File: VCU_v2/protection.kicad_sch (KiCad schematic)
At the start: 8 parts, among them Q1 PMOS

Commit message: bspd schematic done
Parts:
- D7: LCSC P/N (none) -> C99290
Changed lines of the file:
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@@
+			)
+		)
+		(property "LCSC P/N" "C99290"
+			(at 147.32 68.58 90)
+			(effects
+				(font
+					(size 1.27 1.27)
+				)
+				(hide yes)
 			)
 		)

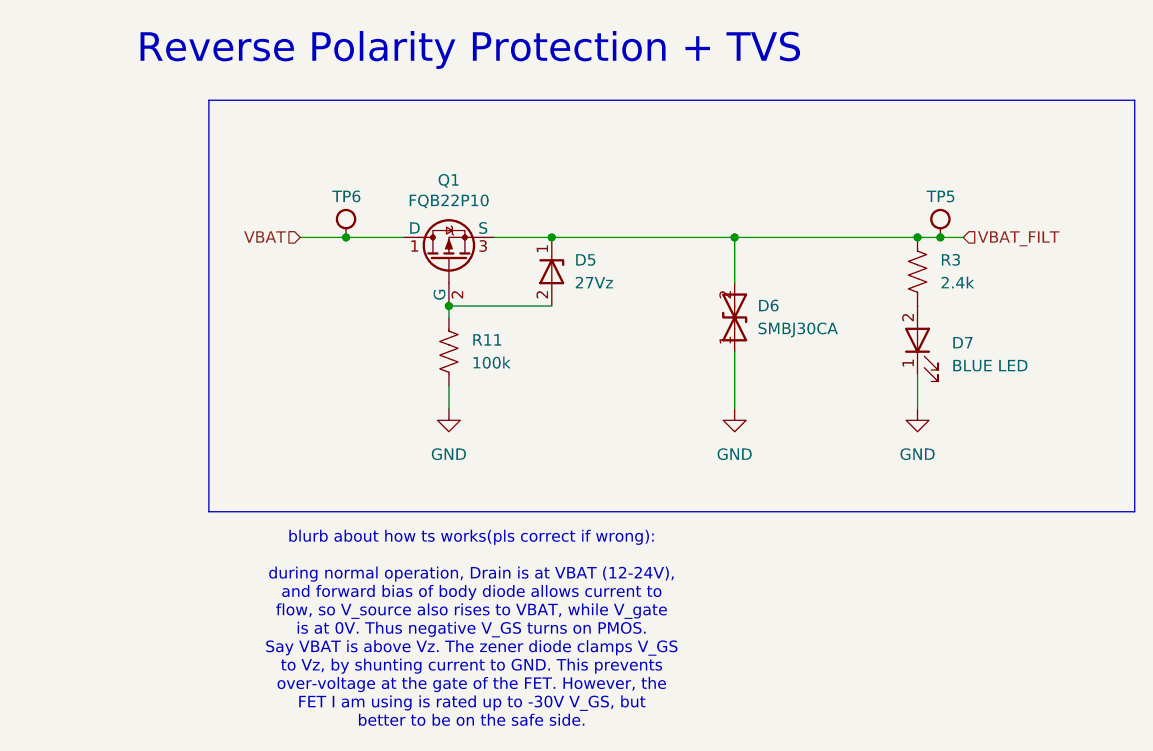
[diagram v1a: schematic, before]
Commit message: vcu v2 schematics done
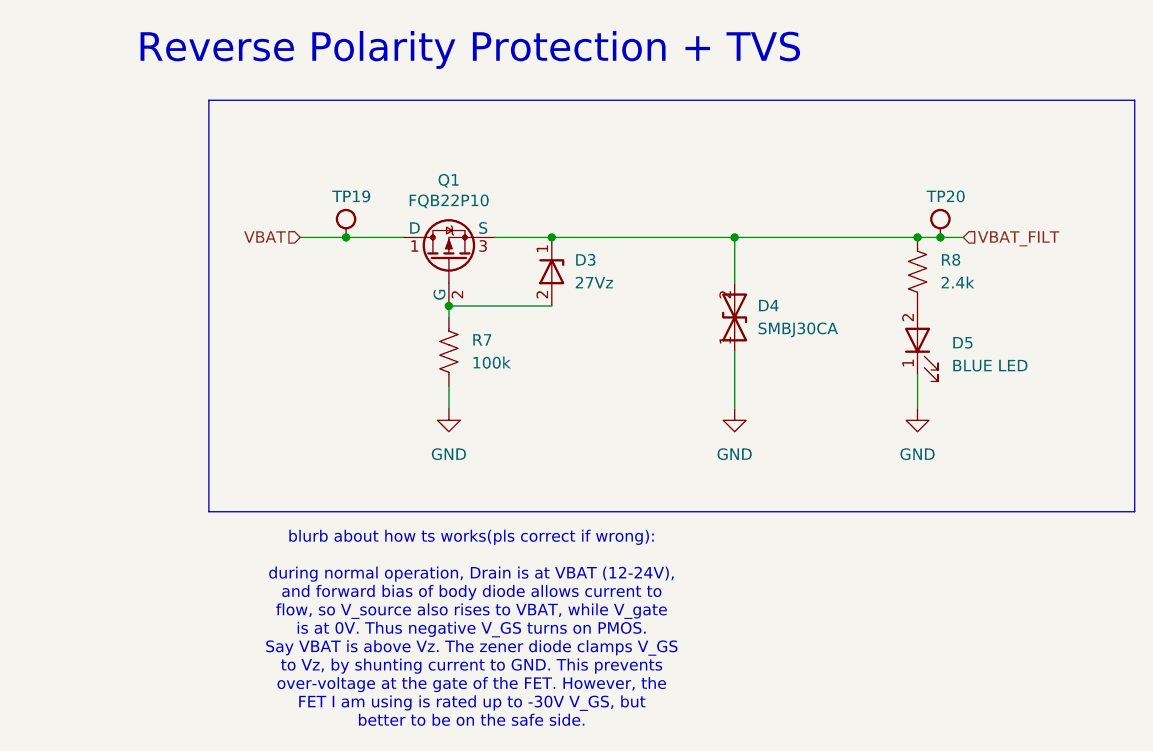
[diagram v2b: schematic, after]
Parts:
- renumbered D5 to D3, D6 to D4, D7 to D5, R11 to R7, R3 to R8, TP6 to TP19, TP5 to TP20
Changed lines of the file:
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@@
 		(dnp no)
 		(fields_autoplaced yes)
-		(property "Reference" "D5"
+		(property "Reference" "D3"
 			(at 109.22 59.6899 90)
 			(effects
@@
 			(project ""
 				(path "/4ee6c2ad-9a1b-4276-b3cf-1cc8dc52967e/9e4b5f8d-93dc-46d5-aa92-d0e0d2e07b3d/b7d8a0a7-c635-4617-919c-9464d63ae6b1"
-					(reference "D5")
+					(reference "D3")
 					(unit 1)
 				)
@@
 		(on_board yes)
 		(dnp no)
-		(property "Reference" "TP5"
+		(property "Reference" "TP20"
 			(at 148.3368 51.8937 0)
 			(effects
@@
 			(project "VCU_v1"
 				(path "/4ee6c2ad-9a1b-4276-b3cf-1cc8dc52967e/9e4b5f8d-93dc-46d5-aa92-d0e0d2e07b3d/b7d8a0a7-c635-4617-919c-9464d63ae6b1"
-					(reference "TP5")
+					(reference "TP20")
 					(unit 1)
 				)
@@
 		(on_board yes)
 		(dnp no)
-		(property "Reference" "TP6"
+		(property "Reference" "TP19"
 			(at 82.2968 51.8937 0)
 			(effects
@@
 			(project "VCU_v1"
 				(path "/4ee6c2ad-9a1b-4276-b3cf-1cc8dc52967e/9e4b5f8d-93dc-46d5-aa92-d0e0d2e07b3d/b7d8a0a7-c635-4617-919c-9464d63ae6b1"
-					(reference "TP6")
+					(reference "TP19")
 					(unit 1)
 				)
@@
 		(dnp no)
 		(fields_autoplaced yes)
-		(property "Reference" "#PWR059"
+		(property "Reference" "#PWR039"
 			(at 127 82.55 0)
 			(effects
@@
 			(project "VCU_v1"
 				(path "/4ee6c2ad-9a1b-4276-b3cf-1cc8dc52967e/9e4b5f8d-93dc-46d5-aa92-d0e0d2e07b3d/b7d8a0a7-c635-4617-919c-9464d63ae6b1"
-					(reference "#PWR059")
+					(reference "#PWR039")
 					(unit 1)
 				)
@@
 		(dnp no)
 		(fields_autoplaced yes)
-		(property "Reference" "D7"
+		(property "Reference" "D5"
 			(at 151.13 68.8974 90)
 			(effects
@@
 			(project ""
 				(path "/4ee6c2ad-9a1b-4276-b3cf-1cc8dc52967e/9e4b5f8d-93dc-46d5-aa92-d0e0d2e07b3d/b7d8a0a7-c635-4617-919c-9464d63ae6b1"
-					(reference "D7")
+					(reference "D5")
 					(unit 1)
 				)
@@
 		(dnp no)
 		(fields_autoplaced yes)
-		(property "Reference" "R11"
+		(property "Reference" "R7"
 			(at 97.79 68.5799 90)
 			(effects
@@
 			(project ""
 				(path "/4ee6c2ad-9a1b-4276-b3cf-1cc8dc52967e/9e4b5f8d-93dc-46d5-aa92-d0e0d2e07b3d/b7d8a0a7-c635-4617-919c-9464d63ae6b1"
-					(reference "R11")
+					(reference "R7")
 					(unit 1)
 				)
@@
 		(dnp no)
 		(fields_autoplaced yes)
-		(property "Reference" "D6"
+		(property "Reference" "D4"
 			(at 129.54 64.7699 90)
 			(effects
@@
 			(project ""
 				(path "/4ee6c2ad-9a1b-4276-b3cf-1cc8dc52967e/9e4b5f8d-93dc-46d5-aa92-d0e0d2e07b3d/b7d8a0a7-c635-4617-919c-9464d63ae6b1"
-					(reference "D6")
+					(reference "D4")
 					(unit 1)
 				)
@@
 		(dnp no)
 		(fields_autoplaced yes)
-		(property "Reference" "#PWR058"
+		(property "Reference" "#PWR038"
 			(at 95.25 82.55 0)
 			(effects
@@
 			(project ""
 				(path "/4ee6c2ad-9a1b-4276-b3cf-1cc8dc52967e/9e4b5f8d-93dc-46d5-aa92-d0e0d2e07b3d/b7d8a0a7-c635-4617-919c-9464d63ae6b1"
-					(reference "#PWR058")
+					(reference "#PWR038")
 					(unit 1)
 				)
@@
 		(dnp no)
 		(fields_autoplaced yes)
-		(property "Reference" "R3"
+		(property "Reference" "R8"
 			(at 149.86 59.6899 90)
 			(effects
@@
 			(project ""
 				(path "/4ee6c2ad-9a1b-4276-b3cf-1cc8dc52967e/9e4b5f8d-93dc-46d5-aa92-d0e0d2e07b3d/b7d8a0a7-c635-4617-919c-9464d63ae6b1"
-					(reference "R3")
+					(reference "R8")
 					(unit 1)
 				)
@@
 		(dnp no)
 		(fields_autoplaced yes)
-		(property "Reference" "#PWR060"
+		(property "Reference" "#PWR040"
 			(at 147.32 82.55 0)
 			(effects
@@
 			(project ""
 				(path "/4ee6c2ad-9a1b-4276-b3cf-1cc8dc52967e/9e4b5f8d-93dc-46d5-aa92-d0e0d2e07b3d/b7d8a0a7-c635-4617-919c-9464d63ae6b1"
-					(reference "#PWR060")
+					(reference "#PWR040")
 					(unit 1)
 				)

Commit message: placements friggin 80% friggin done shoutout epstein
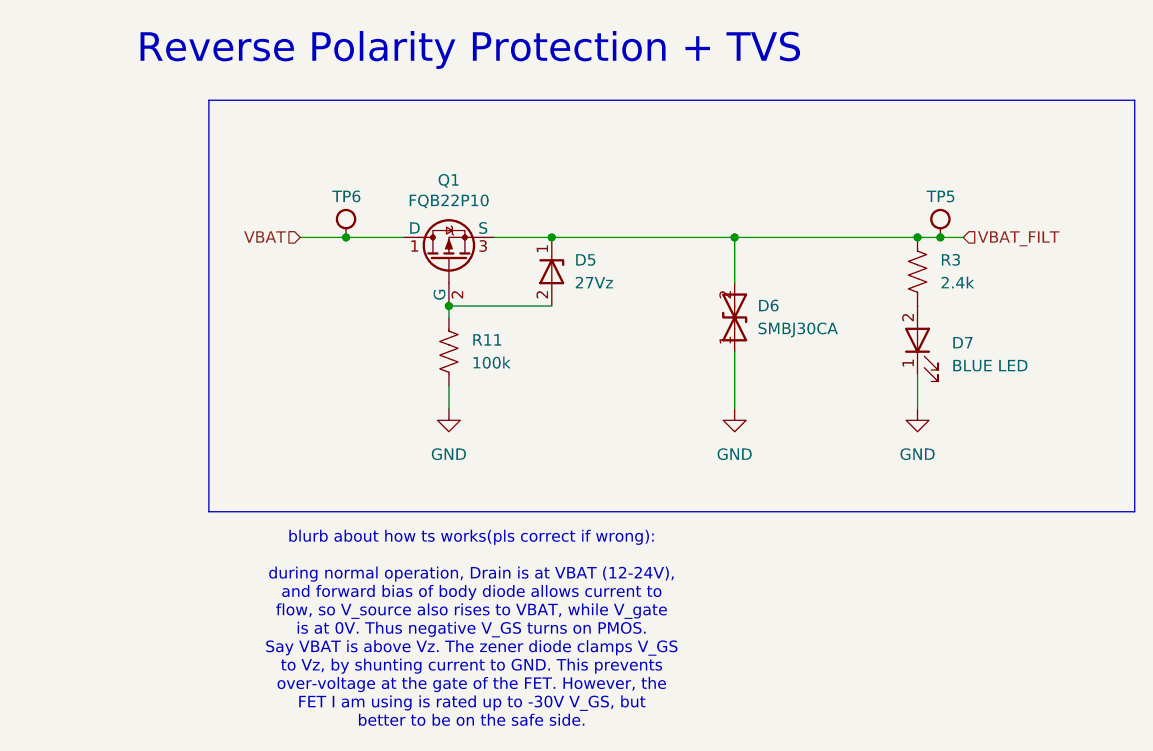
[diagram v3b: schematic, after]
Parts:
- renumbered D3 to D5, D4 to D6, D5 to D7, R7 to R11, R8 to R3, TP20 to TP5, TP19 to TP6
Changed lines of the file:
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@@
 		(dnp no)
 		(fields_autoplaced yes)
-		(property "Reference" "D3"
+		(property "Reference" "D5"
 			(at 109.22 59.6899 90)
 			(effects
@@
 			(project ""
 				(path "/4ee6c2ad-9a1b-4276-b3cf-1cc8dc52967e/9e4b5f8d-93dc-46d5-aa92-d0e0d2e07b3d/b7d8a0a7-c635-4617-919c-9464d63ae6b1"
-					(reference "D3")
+					(reference "D5")
 					(unit 1)
 				)
@@
 		(on_board yes)
 		(dnp no)
-		(property "Reference" "TP20"
+		(property "Reference" "TP5"
 			(at 148.3368 51.8937 0)
 			(effects
@@
 			(project "VCU_v1"
 				(path "/4ee6c2ad-9a1b-4276-b3cf-1cc8dc52967e/9e4b5f8d-93dc-46d5-aa92-d0e0d2e07b3d/b7d8a0a7-c635-4617-919c-9464d63ae6b1"
-					(reference "TP20")
+					(reference "TP5")
 					(unit 1)
 				)
@@
 		(on_board yes)
 		(dnp no)
-		(property "Reference" "TP19"
+		(property "Reference" "TP6"
 			(at 82.2968 51.8937 0)
 			(effects
@@
 			(project "VCU_v1"
 				(path "/4ee6c2ad-9a1b-4276-b3cf-1cc8dc52967e/9e4b5f8d-93dc-46d5-aa92-d0e0d2e07b3d/b7d8a0a7-c635-4617-919c-9464d63ae6b1"
-					(reference "TP19")
+					(reference "TP6")
 					(unit 1)
 				)
@@
 		(dnp no)
 		(fields_autoplaced yes)
-		(property "Reference" "#PWR039"
+		(property "Reference" "#PWR059"
 			(at 127 82.55 0)
 			(effects
@@
 			(project "VCU_v1"
 				(path "/4ee6c2ad-9a1b-4276-b3cf-1cc8dc52967e/9e4b5f8d-93dc-46d5-aa92-d0e0d2e07b3d/b7d8a0a7-c635-4617-919c-9464d63ae6b1"
-					(reference "#PWR039")
+					(reference "#PWR059")
 					(unit 1)
 				)
@@
 		(dnp no)
 		(fields_autoplaced yes)
-		(property "Reference" "D5"
+		(property "Reference" "D7"
 			(at 151.13 68.8974 90)
 			(effects
@@
 			(project ""
 				(path "/4ee6c2ad-9a1b-4276-b3cf-1cc8dc52967e/9e4b5f8d-93dc-46d5-aa92-d0e0d2e07b3d/b7d8a0a7-c635-4617-919c-9464d63ae6b1"
-					(reference "D5")
+					(reference "D7")
 					(unit 1)
 				)
@@
 		(dnp no)
 		(fields_autoplaced yes)
-		(property "Reference" "R7"
+		(property "Reference" "R11"
 			(at 97.79 68.5799 90)
 			(effects
@@
 			(project ""
 				(path "/4ee6c2ad-9a1b-4276-b3cf-1cc8dc52967e/9e4b5f8d-93dc-46d5-aa92-d0e0d2e07b3d/b7d8a0a7-c635-4617-919c-9464d63ae6b1"
-					(reference "R7")
+					(reference "R11")
 					(unit 1)
 				)
@@
 		(dnp no)
 		(fields_autoplaced yes)
-		(property "Reference" "D4"
+		(property "Reference" "D6"
 			(at 129.54 64.7699 90)
 			(effects
@@
 			(project ""
 				(path "/4ee6c2ad-9a1b-4276-b3cf-1cc8dc52967e/9e4b5f8d-93dc-46d5-aa92-d0e0d2e07b3d/b7d8a0a7-c635-4617-919c-9464d63ae6b1"
-					(reference "D4")
+					(reference "D6")
 					(unit 1)
 				)
@@
 		(dnp no)
 		(fields_autoplaced yes)
-		(property "Reference" "#PWR038"
+		(property "Reference" "#PWR058"
 			(at 95.25 82.55 0)
 			(effects
@@
 			(project ""
 				(path "/4ee6c2ad-9a1b-4276-b3cf-1cc8dc52967e/9e4b5f8d-93dc-46d5-aa92-d0e0d2e07b3d/b7d8a0a7-c635-4617-919c-9464d63ae6b1"
-					(reference "#PWR038")
+					(reference "#PWR058")
 					(unit 1)
 				)
@@
 		(dnp no)
 		(fields_autoplaced yes)
-		(property "Reference" "R8"
+		(property "Reference" "R3"
 			(at 149.86 59.6899 90)
 			(effects
@@
 			(project ""
 				(path "/4ee6c2ad-9a1b-4276-b3cf-1cc8dc52967e/9e4b5f8d-93dc-46d5-aa92-d0e0d2e07b3d/b7d8a0a7-c635-4617-919c-9464d63ae6b1"
-					(reference "R8")
+					(reference "R3")
 					(unit 1)
 				)
@@
 		(dnp no)
 		(fields_autoplaced yes)
-		(property "Reference" "#PWR040"
+		(property "Reference" "#PWR060"
 			(at 147.32 82.55 0)
 			(effects
@@
 			(project ""
 				(path "/4ee6c2ad-9a1b-4276-b3cf-1cc8dc52967e/9e4b5f8d-93dc-46d5-aa92-d0e0d2e07b3d/b7d8a0a7-c635-4617-919c-9464d63ae6b1"
-					(reference "#PWR040")
+					(reference "#PWR060")
 					(unit 1)
 				)
